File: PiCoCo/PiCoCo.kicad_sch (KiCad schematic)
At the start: 15 parts, among them IC1 74FST3257DR2G, IC2 74FST3257DR2G, J1 Conn_01x02_Pin, U1 Pico, U2 74HC244, U3 74HC244, U4 74HC244

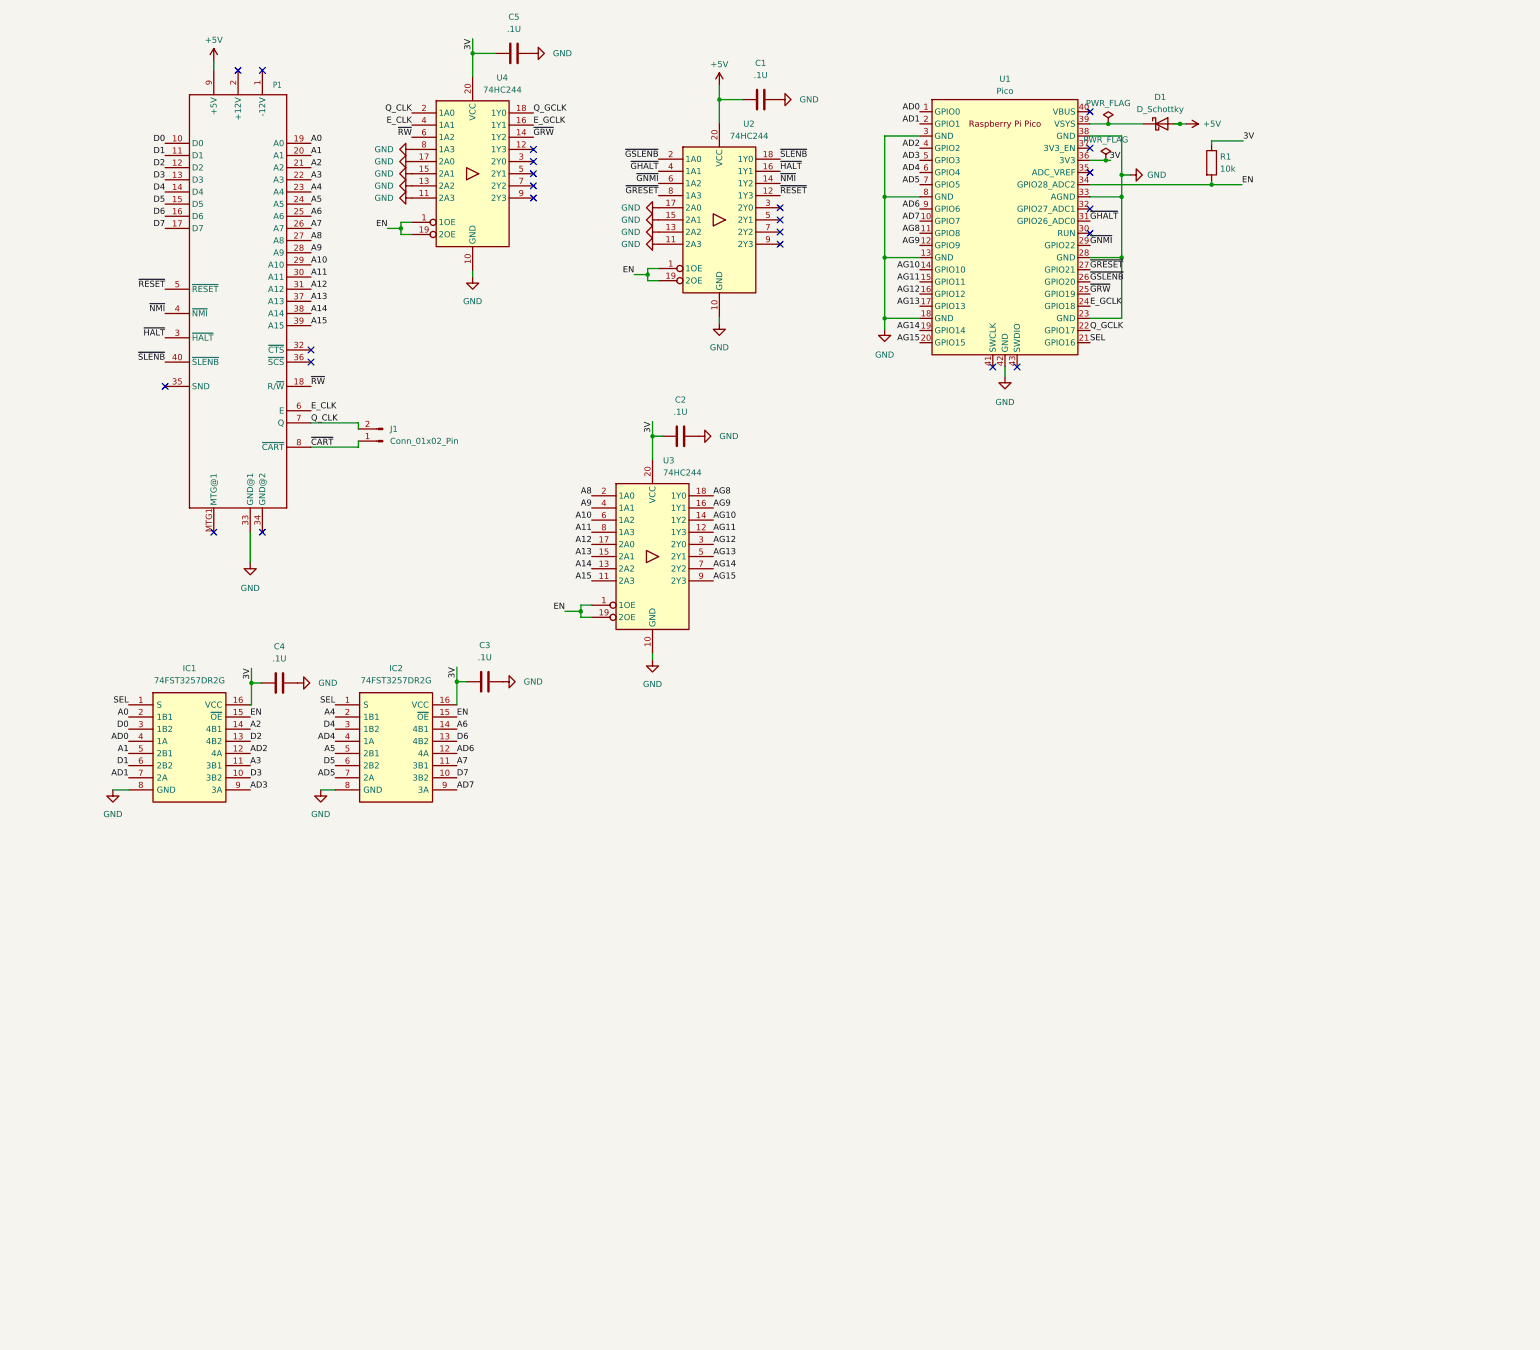
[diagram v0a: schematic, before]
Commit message: Working on hand-testing version
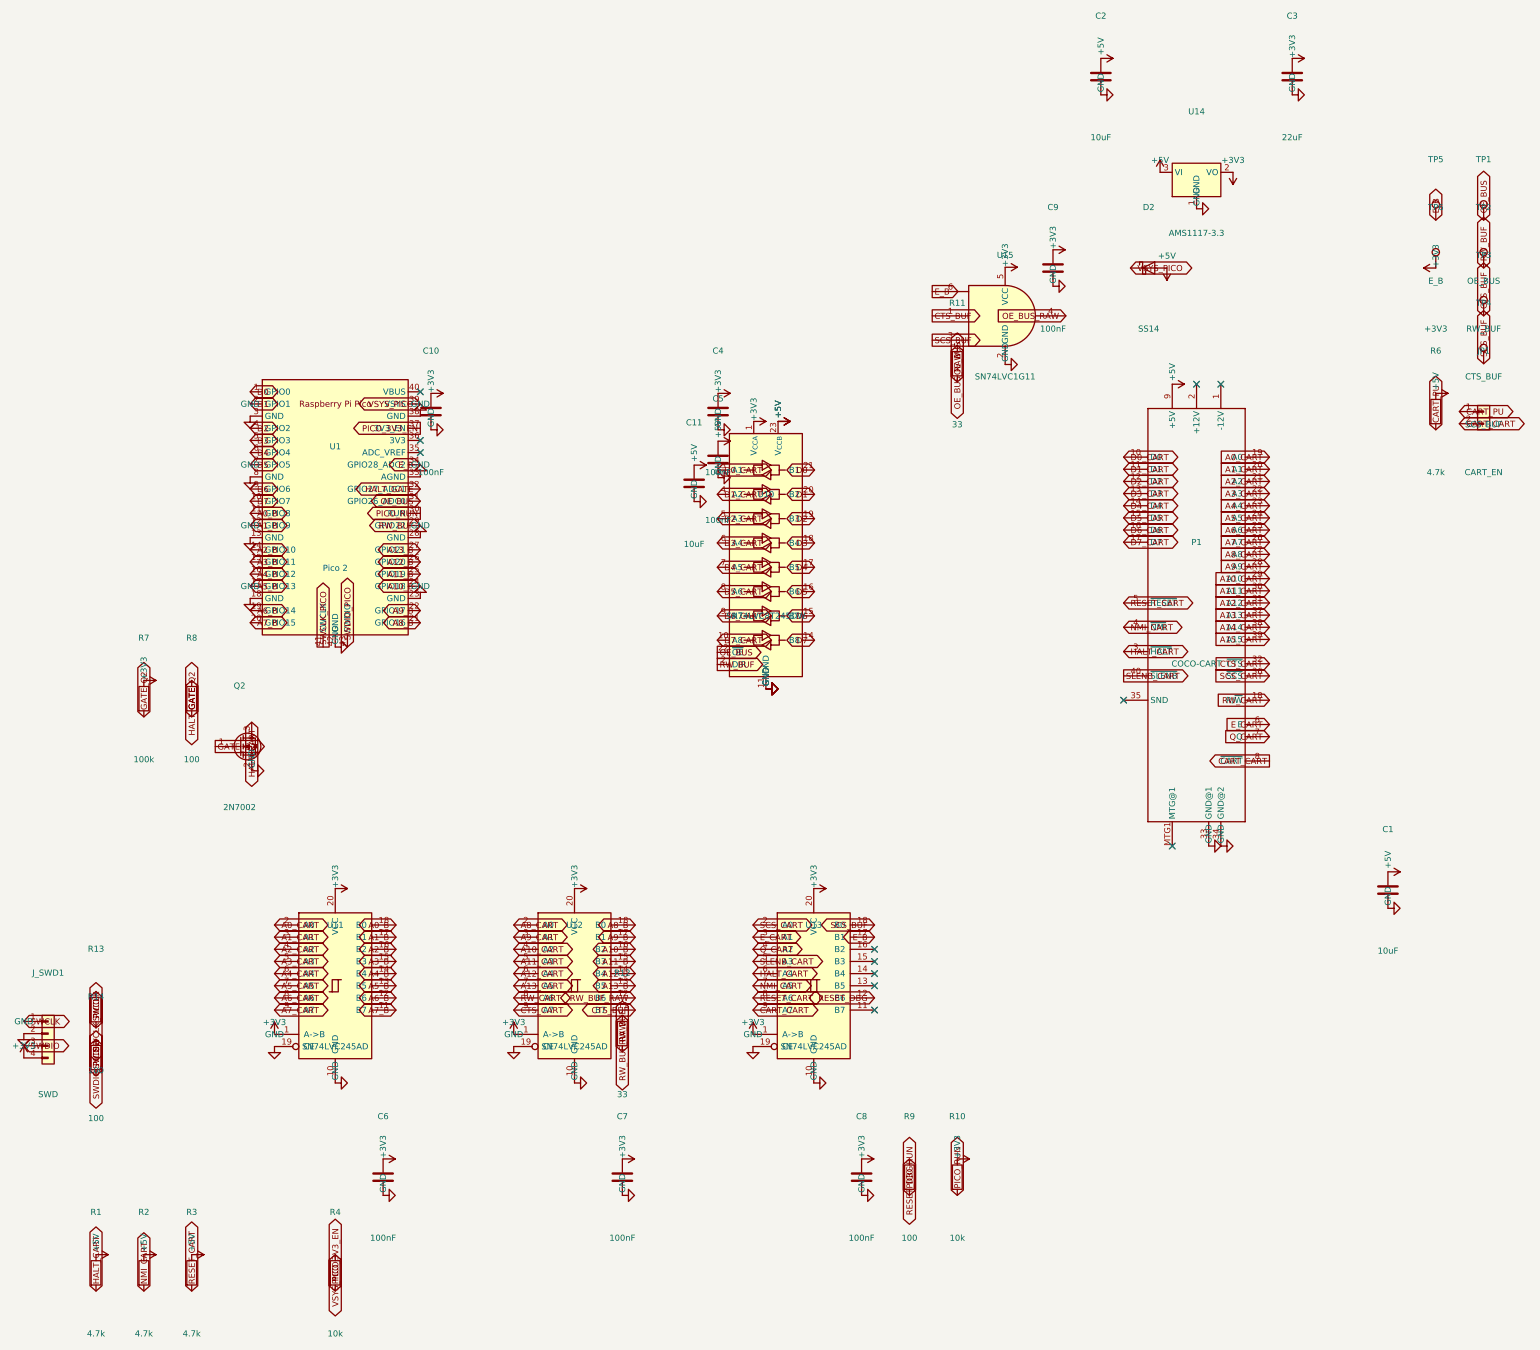
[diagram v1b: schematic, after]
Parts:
- removed D1: D_Schottky, Diode_SMD:D_SOD-123, symbol Device:D_Schottky
- removed IC1, IC2: 74FST3257DR2G, Package_SO:TSSOP-16_4.4x5mm_P0.65mm, symbol PiCoCo:74FST3257DR2G
- removed J1: Conn_01x02_Pin, Connector_PinHeader_2.54mm:PinHeader_1x02_P2.54mm_Vertical, symbol Connector:Conn_01x02_Pin
- removed U2, U3, U4: 74HC244, Package_SO:TSSOP-20_4.4x6.5mm_P0.65mm, symbol 74xx:74HC244
- added C10, C6, C7, C8, C9: 100nF, Capacitor_SMD:C_0805_2012Metric, symbol Device:C
- added C11: 10uF, Capacitor_SMD:C_0805_2012Metric, symbol Device:C
- added D2: SS14, Diode_SMD:D_SMA, symbol Device:D_Schottky
- added JP1: CART_EN, Connector_PinHeader_2.54mm:PinHeader_1x02_P2.54mm_Vertical, symbol Connector_Generic:Conn_01x02
- added J_SWD1: SWD, Connector_PinHeader_2.54mm:PinHeader_1x04_P2.54mm_Vertical, symbol Connector_Generic:Conn_01x04
- added Q2: 2N7002, Package_TO_SOT_SMD:SOT-23, symbol Transistor_FET:Q_NMOS_GSD
- added R10, R4: 10k, Resistor_SMD:R_0805_2012Metric, symbol Device:R
- added R11, R12: 33, Resistor_SMD:R_0805_2012Metric, symbol Device:R
- added R13, R14, R8, R9: 100, Resistor_SMD:R_0805_2012Metric, symbol Device:R
- added R2, R3, R6: 4.7k, Resistor_SMD:R_0805_2012Metric, symbol Device:R
- added R7: 100k, Resistor_SMD:R_0805_2012Metric, symbol Device:R
- added TP1: OE_BUS, TestPoint:TestPoint_Pad_1.0x1.0mm, symbol Connector:TestPoint
- added TP2: RW_BUF, TestPoint:TestPoint_Pad_1.0x1.0mm, symbol Connector:TestPoint
- added TP3: CTS_BUF, TestPoint:TestPoint_Pad_1.0x1.0mm, symbol Connector:TestPoint
- added TP4: SCS_BUF, TestPoint:TestPoint_Pad_1.0x1.0mm, symbol Connector:TestPoint
- added TP5: E_B, TestPoint:TestPoint_Pad_1.0x1.0mm, symbol Connector:TestPoint
- added TP6: +3V3, TestPoint:TestPoint_Pad_1.0x1.0mm, symbol Connector:TestPoint
- added U10: SN74LVC8T245DW, Package_SO:SOIC-24W_7.5x15.4mm_P1.27mm, symbol Logic_LevelTranslator:SN74LVC8T245
- added U11, U12, U13: SN74LVC245AD, Package_SO:SOIC-20W_7.5x12.8mm_P1.27mm, symbol 74xx:74LS245
- added U14: AMS1117-3.3, Package_TO_SOT_SMD:SOT-223-3_TabPin2, symbol Regulator_Linear:AP1117-15
- added U15: SN74LVC1G11, Package_TO_SOT_SMD:SOT-363_SC-70-6, symbol 74xGxx:74LVC1G11
- C1, C2: value .1U -> 10uF; footprint Capacitor_SMD:C_0805_2012Metric_Pad1.18x1.45mm_HandSolder -> Capacitor_SMD:C_0805_2012Metric
- C3: value .1U -> 22uF; footprint Capacitor_SMD:C_0805_2012Metric_Pad1.18x1.45mm_HandSolder -> Capacitor_SMD:C_0805_2012Metric
- C4, C5: value .1U -> 100nF; footprint Capacitor_SMD:C_0805_2012Metric_Pad1.18x1.45mm_HandSolder -> Capacitor_SMD:C_0805_2012Metric
- P1: value ~ -> COCO-CART
- R1: value 10k -> 4.7k; footprint Resistor_SMD:R_0805_2012Metric_Pad1.20x1.40mm_HandSolder -> Resistor_SMD:R_0805_2012Metric
- U1: value Pico -> Pico 2
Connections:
- net AD0 is gone; now on net D0: U1.1 (GPIO0)
- net AD1 is gone; now on net D1: U1.2 (GPIO1)
- net AD2 is gone; now on net D2: U1.4 (GPIO2)
- net AD3 is gone; now on net D3: U1.5 (GPIO3)
- net AD4 is gone; now on net D4: U1.6 (GPIO4)
- net AD5 is gone; now on net D5: U1.7 (GPIO5)
- net AD6 is gone; now on net D6: U1.9 (GPIO6)
- net AD7 is gone; now on net D7: U1.10 (GPIO7)
- net +5V: now also C1.1, C2.1, C5.1, R1.1, C11.1, D2.2 (A), R2.1, R3.1, R6.1, U10.23 (V_{CCB}), U10.24 (V_{CCB}), U14.3 (VI); no longer C1.2
- net D0: now also U10.21 (B1); no longer P1.10 (D0)
- net D1: now also U10.20 (B2); no longer P1.11 (D1)
- net D2: now also U10.19 (B3); no longer P1.12 (D2)
- net D3: now also U10.18 (B4); no longer P1.13 (D3)
- net D4: now also U10.17 (B5); no longer P1.14 (D4)
- net D5: now also U10.16 (B6); no longer P1.15 (D5)
- net D6: now also U10.15 (B7); no longer P1.16 (D6)
- net D7: now also U10.14 (B8); no longer P1.17 (D7)
- net GND: now also C1.2, C2.2, C3.2, C4.2, C5.2, P1.34 (GND@2), C10.2, C11.2, C6.2, C7.2, C8.2, C9.2, J_SWD1.2 (Pin_2), Q2.2 (S), U10.11 (GND), U10.12 (GND), U10.13 (GND), U11.10 (GND), U11.19 (CE), U12.10 (GND), U12.19 (CE), U13.10 (GND), U13.19 (CE), U14.1 (GND), U15.2 (GND); no longer C1.1, C2.1, C3.1, C4.1, C5.1
- net CTS_CART: now reaches P1.32 (~{CTS})
- net CTS_CART: now also U12.9 (A7)
- net SCS_CART: now reaches P1.36 (~{SCS})
- net SCS_CART: now also U13.2 (A0)
- net PICO_RUN: now reaches U1.30 (RUN)
- net PICO_RUN: now also R10.2, R9.2
- net HALT_GATE: now reaches U1.32 (GPIO27_ADC1)
- net HALT_GATE: now also R8.1
- net PICO_3V3_EN: now reaches U1.37 (3V3_EN)
- net PICO_3V3_EN: now also R4.2
- net VSYS_PICO: now reaches U1.39 (VSYS)
- net VSYS_PICO: now also D2.1 (K), R4.1
- net SWCLK_PICO: now reaches U1.41 (SWCLK)
- net SWCLK_PICO: now also R13.1
- net SWDIO_PICO: now reaches U1.43 (SWDIO)
- net SWDIO_PICO: now also R14.1
- removed net 3V: C2.2, C3.2, C4.2, C5.2, R1.1, U1.36 (3V3)
- net A0 renamed A0_CART
- net A0_CART: now also U11.2 (A0)
- net A1 renamed A1_CART
- net A1_CART: now also U11.3 (A1)
- net A10 renamed A10_CART
- net A10_CART: now also U12.4 (A2)
- net A11 renamed A11_CART
- net A11_CART: now also U12.5 (A3)
- net A12 renamed A12_CART
- net A12_CART: now also U12.6 (A4)
- net A13 renamed A13_CART
- net A13_CART: now also U12.7 (A5)
- net A14 renamed A14_CART
- net A15 renamed A15_CART
- net A2 renamed A2_CART
- net A2_CART: now also U11.4 (A2)
- net A3 renamed A3_CART
- net A3_CART: now also U11.5 (A3)
- net A4 renamed A4_CART
- net A4_CART: now also U11.6 (A4)
- net A5 renamed A5_CART
- net A5_CART: now also U11.7 (A5)
- net A6 renamed A6_CART
- net A6_CART: now also U11.8 (A6)
- net A7 renamed A7_CART
- net A7_CART: now also U11.9 (A7)
- net A8 renamed A8_CART
- net A8_CART: now also U12.2 (A0)
- net A9 renamed A9_CART
- net A9_CART: now also U12.3 (A1)
- net AG10 renamed A2_B
- net A2_B: now also U11.16 (B2)
- net AG11 renamed A3_B
- net A3_B: now also U11.15 (B3)
- net AG12 renamed A4_B
- net A4_B: now also U11.14 (B4)
- net AG13 renamed A5_B
- net A5_B: now also U11.13 (B5)
- net AG14 renamed A6_B
- net A6_B: now also U11.12 (B6)
- net AG15 renamed A7_B
- net A7_B: now also U11.11 (B7)
- net AG8 renamed A0_B
- net A0_B: now also U11.18 (B0)
- net AG9 renamed A1_B
- net A1_B: now also U11.17 (B1)
- net EN renamed E_B
- net E_B: now also TP5.1, U13.17 (B1), U15.6; no longer R1.2
- net E_CLK renamed E_CART
- net E_CART: now also U13.3 (A1)
- net E_GCLK renamed A10_B
- net A10_B: now also U12.16 (B2)
- net Q_CLK renamed Q_CART
- net Q_CART: now also U13.4 (A2)
- net Q_GCLK renamed A9_B
- net A9_B: now also U12.17 (B1)
- net SEL renamed A8_B
- net A8_B: now also U12.18 (B0)
- net ~{CART} renamed CART_CART
- net CART_CART: now also JP1.2 (Pin_2), U13.9 (A7)
- net ~{GHALT} renamed OE_BUS
- net OE_BUS: now also R11.2, TP1.1, U10.22 (~{OE})
- net ~{GNMI} renamed RW_BUF
- net RW_BUF: now also R12.2, TP2.1, U10.2 (DIR)
- net ~{GRESET} renamed A13_B
- net A13_B: now also U12.13 (B5)
- net ~{GRW} renamed A11_B
- net A11_B: now also U12.15 (B3)
- net ~{GSLENB} renamed A12_B
- net A12_B: now also U12.14 (B4)
- net ~{HALT} renamed HALT_CART
- net HALT_CART: now also R1.2, Q2.3 (D), U13.6 (A4)
- net ~{NMI} renamed NMI_CART
- net NMI_CART: now also R2.2, U13.7 (A5)
- net ~{RESET} renamed RESET_CART
- net RESET_CART: now also R3.2, U13.8 (A6)
- net ~{RW} renamed RW_CART
- net RW_CART: now also U12.8 (A6)
- net ~{SLENB} renamed SLENB_CART
- net SLENB_CART: now also U13.5 (A3)
- new net +3V3: C10.1, C3.1, C4.1, C6.1, C7.1, C8.1, C9.1, J_SWD1.4 (Pin_4), R10.1, R7.1, TP6.1, U10.1 (V_{CCA}), U11.1 (A->B), U11.20 (VCC), U12.1 (A->B), U12.20 (VCC), U13.1 (A->B), U13.20 (VCC), U14.2 (VO), U15.5 (VCC)
- new net CART_PU: JP1.1 (Pin_1), R6.2
- new net CTS_BUF: TP3.1, U12.11 (B7), U15.1
- new net D0_CART: P1.10 (D0), U10.3 (A1)
- new net D1_CART: P1.11 (D1), U10.4 (A2)
- new net D2_CART: P1.12 (D2), U10.5 (A3)
- new net D3_CART: P1.13 (D3), U10.6 (A4)
- new net D4_CART: P1.14 (D4), U10.7 (A5)
- new net D5_CART: P1.15 (D5), U10.8 (A6)
- new net D6_CART: P1.16 (D6), U10.9 (A7)
- new net D7_CART: P1.17 (D7), U10.10 (A8)
- new net GATE_Q2: Q2.1 (G), R7.2, R8.2
- new net OE_BUS_RAW: R11.1, U15.4
- new net RESET_DBG: R9.1, U13.12 (B6)
- new net RW_BUF_RAW: R12.1, U12.12 (B6)
- new net SCS_BUF: TP4.1, U13.18 (B0), U15.3
- new net SWCLK: J_SWD1.1 (Pin_1), R13.2
- new net SWDIO: J_SWD1.3 (Pin_3), R14.2
- no-connect marks 23 -> 12
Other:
- company: Author: Nathan Byrd -> Nathan Byrd
- title: PiCoCo -> PiCoCo - Pi Pico 2 to Tandy CoCo Cartridge
